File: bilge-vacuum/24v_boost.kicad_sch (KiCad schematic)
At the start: 21 parts, among them Q3 PSMN014-80YL, Q4 PSMN014-80YL, U3 LTC3786

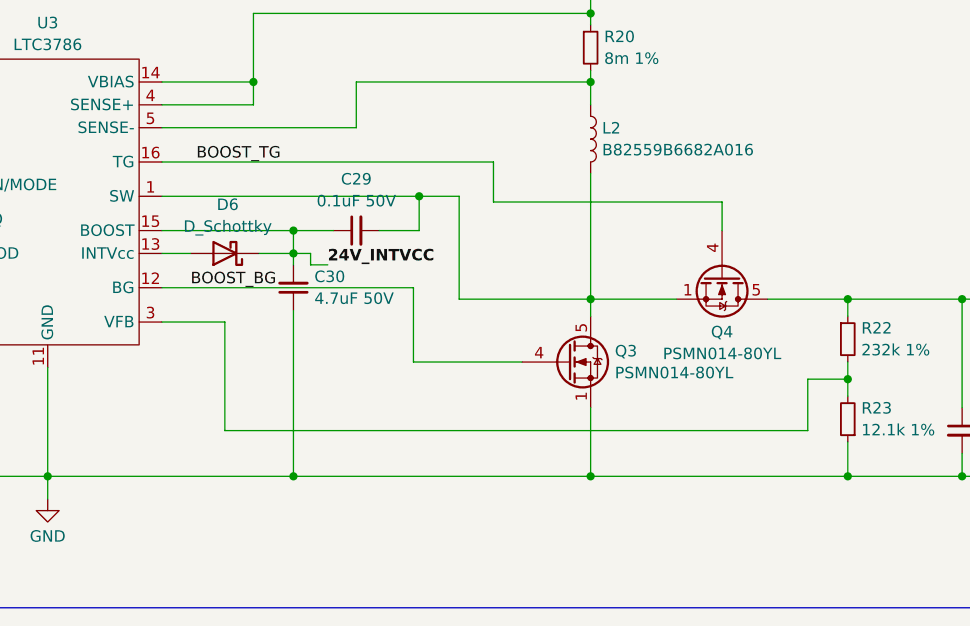
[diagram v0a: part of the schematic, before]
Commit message: Fixes
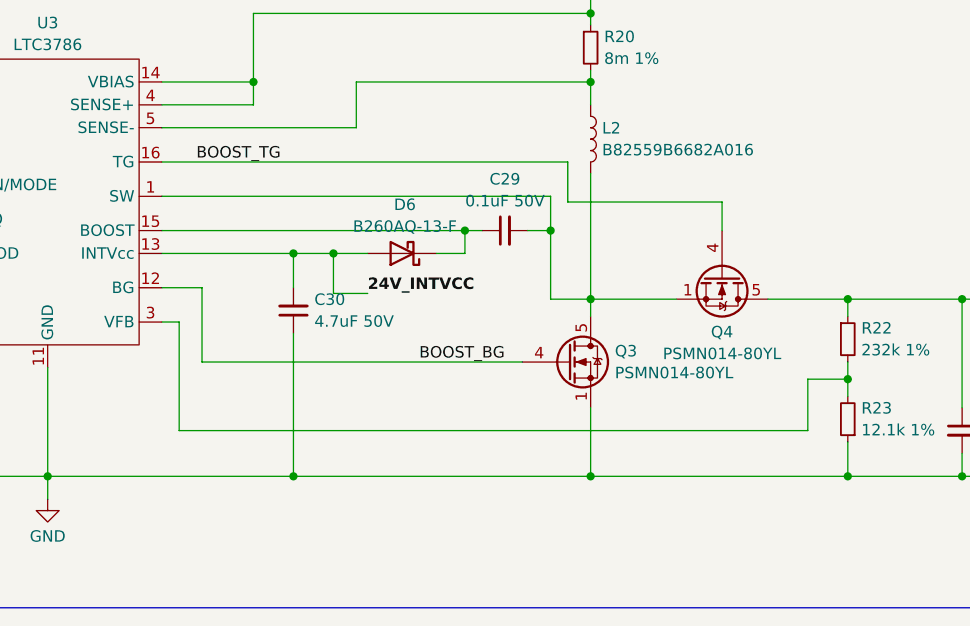
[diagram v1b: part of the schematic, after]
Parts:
- D6: value D_Schottky -> B260AQ-13-F
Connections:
- net 24V_INTVCC: now also D6.2 (A), U3.13 (INTVcc); no longer C29.1, D6.1 (K), U3.15 (BOOST)
- new net: C29.1, D6.1 (K), U3.15 (BOOST)
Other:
- moved on the sheet: C29, C30, D6
